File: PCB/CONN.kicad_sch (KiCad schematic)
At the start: 20 parts, among them J1 mot0, J10 encoder3, J2 encoder0, J3 spare_pins, J4 UART0 DEBUG, J5 mot1, J6 encoder1, J7 mot2, J8 encoder2, J9 mot3, U2 LDL1117_SOT223, U5 USBLC6-2SC6

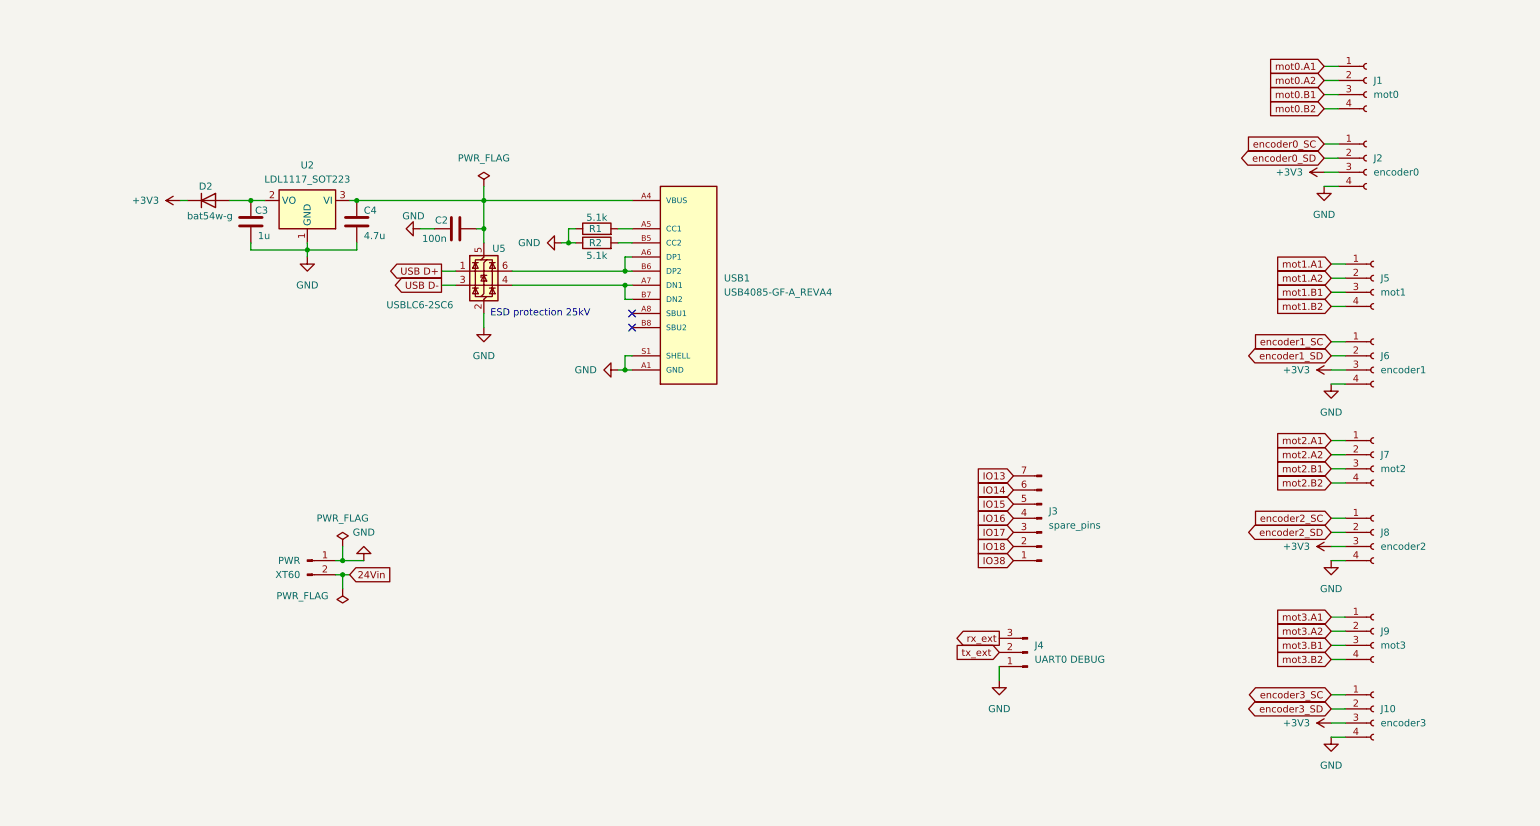
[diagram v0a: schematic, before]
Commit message: PCB layout v1.0
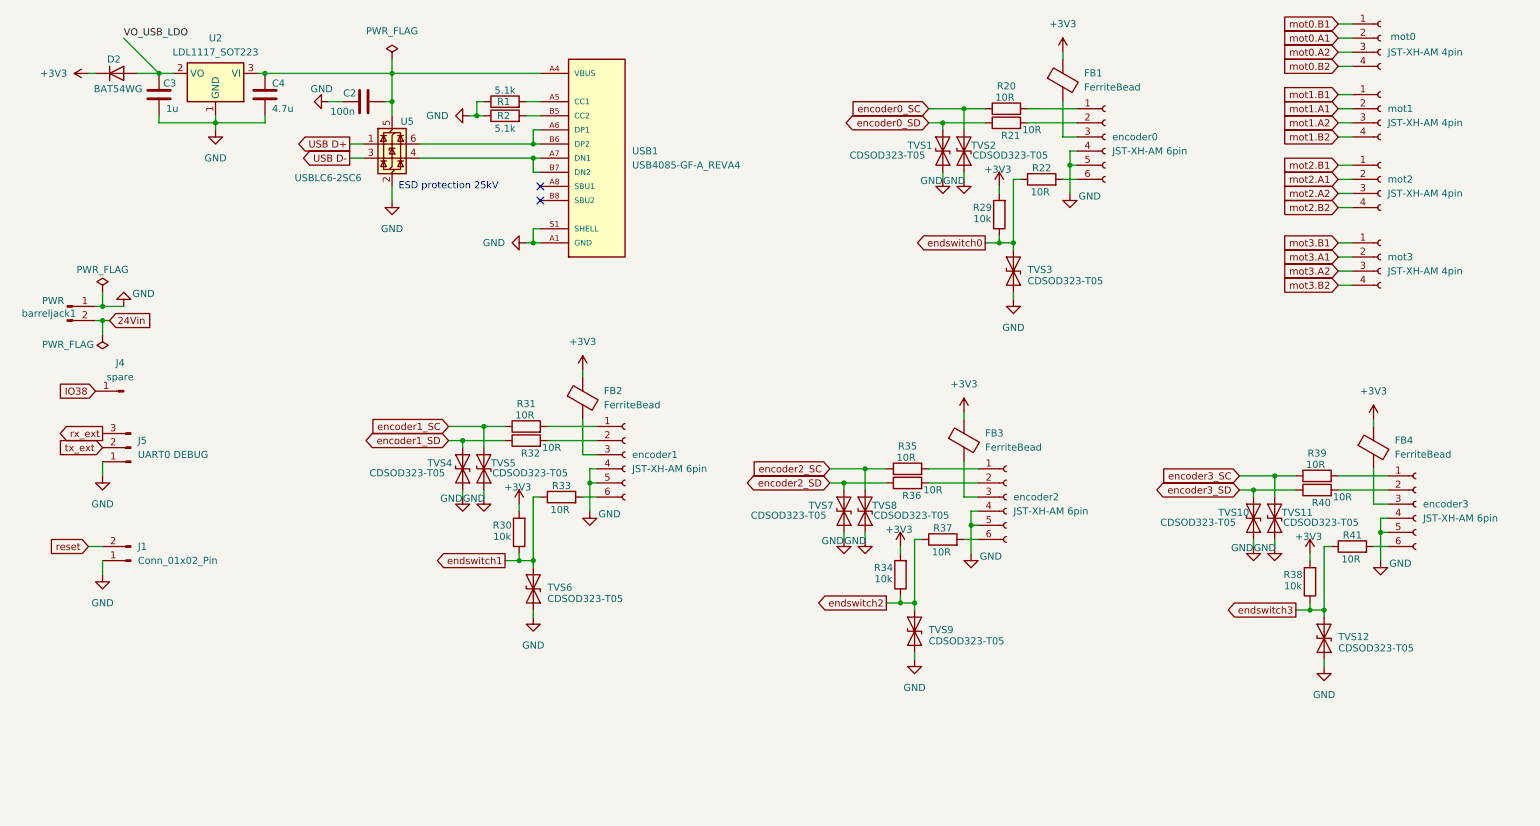
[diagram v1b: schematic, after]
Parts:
- removed J10: encoder3, symbol Connector:Conn_01x04_Socket
- removed J2: encoder0, symbol Connector:Conn_01x04_Socket
- removed J3: spare_pins, symbol Connector:Conn_01x07_Pin
- removed J6: encoder1, symbol Connector:Conn_01x04_Socket
- removed J8: encoder2, symbol Connector:Conn_01x04_Socket
- added FB1, FB2, FB3, FB4: FerriteBead, Inductor_SMD:L_0603_1608Metric_Pad1.05x0.95mm_HandSolder, symbol Device:FerriteBead
- added J1: Conn_01x02_Pin, Connector_PinHeader_2.54mm:PinHeader_1x02_P2.54mm_Vertical, symbol Connector:Conn_01x02_Pin
- added J4: spare, Connector_PinHeader_2.54mm:PinHeader_1x01_P2.54mm_Vertical, symbol Connector:Conn_01x01_Pin
- added R20, R21, R22, R31, R32, R33, R35, R36, R37, R39, R40, R41: 10R, Resistor_SMD:R_0603_1608Metric_Pad0.98x0.95mm_HandSolder, symbol Device:R
- added R29, R30, R34, R38: 10k, Resistor_SMD:R_0603_1608Metric_Pad0.98x0.95mm_HandSolder, symbol Device:R
- added TVS1, TVS10, TVS11, TVS12, TVS2, TVS3, TVS4, TVS5, TVS6, TVS7, TVS8, TVS9: CDSOD323-T05, Diode_SMD:D_SOD-323, symbol Diode:SD05_SOD323
- added encoder0, encoder1, encoder2, encoder3: JST-XH-AM 6pin, Connector_JST:JST_XH_B6B-XH-AM_1x06_P2.50mm_Vertical, symbol Connector:Conn_01x06_Socket
- C2: footprint Capacitor_SMD:C_0201_0603Metric_Pad0.64x0.40mm_HandSolder -> Capacitor_SMD:C_0603_1608Metric_Pad1.08x0.95mm_HandSolder
- C3, C4: footprint (none) -> Capacitor_SMD:C_0603_1608Metric_Pad1.08x0.95mm_HandSolder
- D2: value bat54w-g -> BAT54WG; footprint (none) -> Package_TO_SOT_SMD:SOT-323_SC-70_Handsoldering
- J5: renamed from J4; footprint (none) -> Connector_PinHeader_2.54mm:PinHeader_1x03_P2.54mm_Vertical
- USB1: footprint USB4085-GF-A_REVA4:GCT_USB4085-GF-A_REVA4 -> VNfootprints:GCT_USB4085-GF-A_REVA4
- barreljack1: renamed from XT60; footprint (none) -> Connector_BarrelJack:BarrelJack_CUI_PJ-063AH_Horizontal
- mot0: renamed from J1; value mot0 -> JST-XH-AM 4pin; footprint (none) -> Connector_JST:JST_XH_B4B-XH-AM_1x04_P2.50mm_Vertical
- mot1: renamed from J5; value mot1 -> JST-XH-AM 4pin; footprint (none) -> Connector_JST:JST_XH_B4B-XH-AM_1x04_P2.50mm_Vertical
- mot2: renamed from J7; value mot2 -> JST-XH-AM 4pin; footprint (none) -> Connector_JST:JST_XH_B4B-XH-AM_1x04_P2.50mm_Vertical
- mot3: renamed from J9; value mot3 -> JST-XH-AM 4pin; footprint (none) -> Connector_JST:JST_XH_B4B-XH-AM_1x04_P2.50mm_Vertical
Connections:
- net +3V3: now also FB1.1, FB2.1, FB3.1, FB4.1, R29.2, R30.2, R34.2, R38.2
- net GND: now also J1.1 (Pin_1), TVS1.1 (A1), TVS10.1 (A1), TVS11.1 (A1), TVS12.1 (A1), TVS2.1 (A1), TVS3.1 (A1), TVS4.1 (A1), TVS5.1 (A1), TVS6.1 (A1), TVS7.1 (A1), TVS8.1 (A1), TVS9.1 (A1), encoder0.4 (Pin_4), encoder0.5 (Pin_5), encoder1.4 (Pin_4), encoder1.5 (Pin_5), encoder2.4 (Pin_4), encoder2.5 (Pin_5), encoder3.4 (Pin_4), encoder3.5 (Pin_5)
- net IO38: now also J4.1 (Pin_1)
- net encoder0_SC: now also R20.1, TVS2.2 (A2)
- net encoder0_SD: now also R21.1, TVS1.2 (A2)
- net encoder1_SC: now also R31.1, TVS5.2 (A2)
- net encoder1_SD: now also R32.1, TVS4.2 (A2)
- net encoder2_SC: now also R35.1, TVS8.2 (A2)
- net encoder2_SD: now also R36.1, TVS7.2 (A2)
- net encoder3_SC: now also R39.1, TVS11.2 (A2)
- net encoder3_SD: now also R40.1, TVS10.2 (A2)
- net mot0.A1: now also mot0.2 (Pin_2); no longer mot0.1 (Pin_1)
- net mot0.A2: now also mot0.3 (Pin_3); no longer mot0.2 (Pin_2)
- net mot0.B1: now also mot0.1 (Pin_1); no longer mot0.3 (Pin_3)
- net mot1.A1: now also mot1.2 (Pin_2); no longer mot1.1 (Pin_1)
- net mot1.A2: now also mot1.3 (Pin_3); no longer mot1.2 (Pin_2)
- net mot1.B1: now also mot1.1 (Pin_1); no longer mot1.3 (Pin_3)
- net mot2.A1: now also mot2.2 (Pin_2); no longer mot2.1 (Pin_1)
- net mot2.A2: now also mot2.3 (Pin_3); no longer mot2.2 (Pin_2)
- net mot2.B1: now also mot2.1 (Pin_1); no longer mot2.3 (Pin_3)
- net mot3.A1: now also mot3.2 (Pin_2); no longer mot3.1 (Pin_1)
- net mot3.A2: now also mot3.3 (Pin_3); no longer mot3.2 (Pin_2)
- net mot3.B1: now also mot3.1 (Pin_1); no longer mot3.3 (Pin_3)
- net VO_USB_LDO: now reaches C3.1, D2.2 (A), U2.2 (VO)
- new net: R33.2, encoder1.6 (Pin_6)
- new net: FB4.2, encoder3.3 (Pin_3)
- new net: R21.2, encoder0.2 (Pin_2)
- new net: R22.2, encoder0.6 (Pin_6)
- new net: R20.2, encoder0.1 (Pin_1)
- new net: R41.2, encoder3.6 (Pin_6)
- new net: FB2.2, encoder1.3 (Pin_3)
- new net: R31.2, encoder1.1 (Pin_1)
- new net: R39.2, encoder3.1 (Pin_1)
- new net: R32.2, encoder1.2 (Pin_2)
- new net: R36.2, encoder2.2 (Pin_2)
- new net: R40.2, encoder3.2 (Pin_2)
- new net: R37.2, encoder2.6 (Pin_6)
- new net: R35.2, encoder2.1 (Pin_1)
- new net: FB1.2, encoder0.3 (Pin_3)
- new net: FB3.2, encoder2.3 (Pin_3)
- new net endswitch0: R22.1, R29.1, TVS3.2 (A2)
- new net endswitch1: R30.1, R33.1, TVS6.2 (A2)
- new net endswitch2: R34.1, R37.1, TVS9.2 (A2)
- new net endswitch3: R38.1, R41.1, TVS12.2 (A2)
- new net reset: J1.2 (Pin_2)
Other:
- moved on the sheet: C2, C3, C4, D2, J5, R1, R2, U2, U5, USB1, barreljack1, mot0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

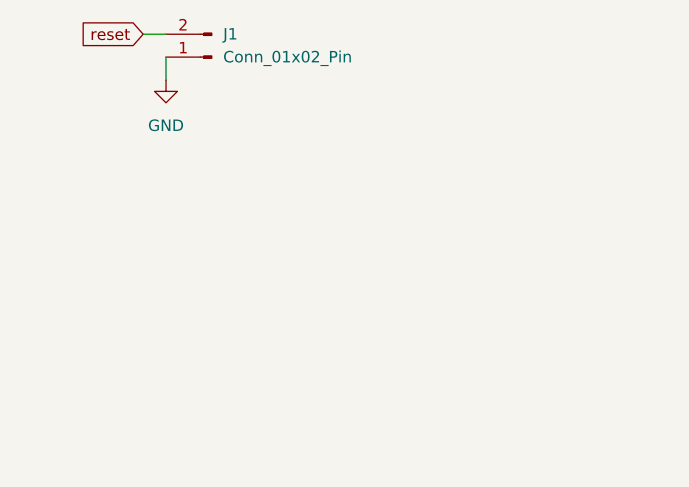
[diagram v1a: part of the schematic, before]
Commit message: pcb version ready for final check
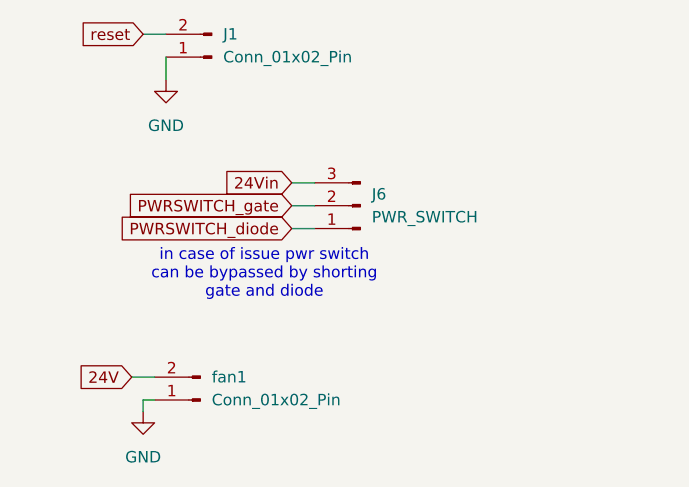
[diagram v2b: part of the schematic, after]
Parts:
- added J6: PWR_SWITCH, Connector_PinHeader_2.54mm:PinHeader_1x03_P2.54mm_Vertical, symbol Connector:Conn_01x03_Pin
- added fan1: Conn_01x02_Pin, Connector_PinHeader_2.54mm:PinHeader_1x02_P2.54mm_Vertical, symbol Connector:Conn_01x02_Pin
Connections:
- net 24Vin: now also J6.3 (Pin_3)
- net GND: now also fan1.1 (Pin_1)
- new net 24V: fan1.2 (Pin_2)
- new net PWRSWITCH_diode: J6.1 (Pin_1)
- new net PWRSWITCH_gate: J6.2 (Pin_2)
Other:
- note added: "in case of issue pwr switch can be bypassed by shorting gate and diode"
